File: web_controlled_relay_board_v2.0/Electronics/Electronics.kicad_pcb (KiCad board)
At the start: 2 copper layers, 165.2 x 114.6 mm, 71 parts, among them J1 Screw_Terminal_01x10, J2 Screw_Terminal_01x10, J3 Screw_Terminal_01x02, J4 Screw_Terminal_01x02, K1 G3MB-202P, K10 G3MB-202P, K11 G3MB-202P, K12 G3MB-202P, K13 G3MB-202P, K14 G3MB-202P, K15 G3MB-202P, K16 G3MB-202P, K17 G3MB-202P, K18 G3MB-202P, K19 G3MB-202P, K2 G3MB-202P, K20 G3MB-202P, K3 G3MB-202P, K4 G3MB-202P, K5 G3MB-202P, K6 G3MB-202P, K7 G3MB-202P, K8 G3MB-202P, K9 G3MB-202P, SW1 SW_MEC_5E, U1 PC817, U10 PC817, U11 PC817, U12 PC817, U13 PC817, U14 PC817, U15 PC817, U16 PC817, U17 PC817, U18 PC817, U19 PC817, U2 PC817, U20 PC817, U3 PC817, U4 PC817, U5 PC817, U6 PC817, U7 PC817, U8 PC817, U9 PC817

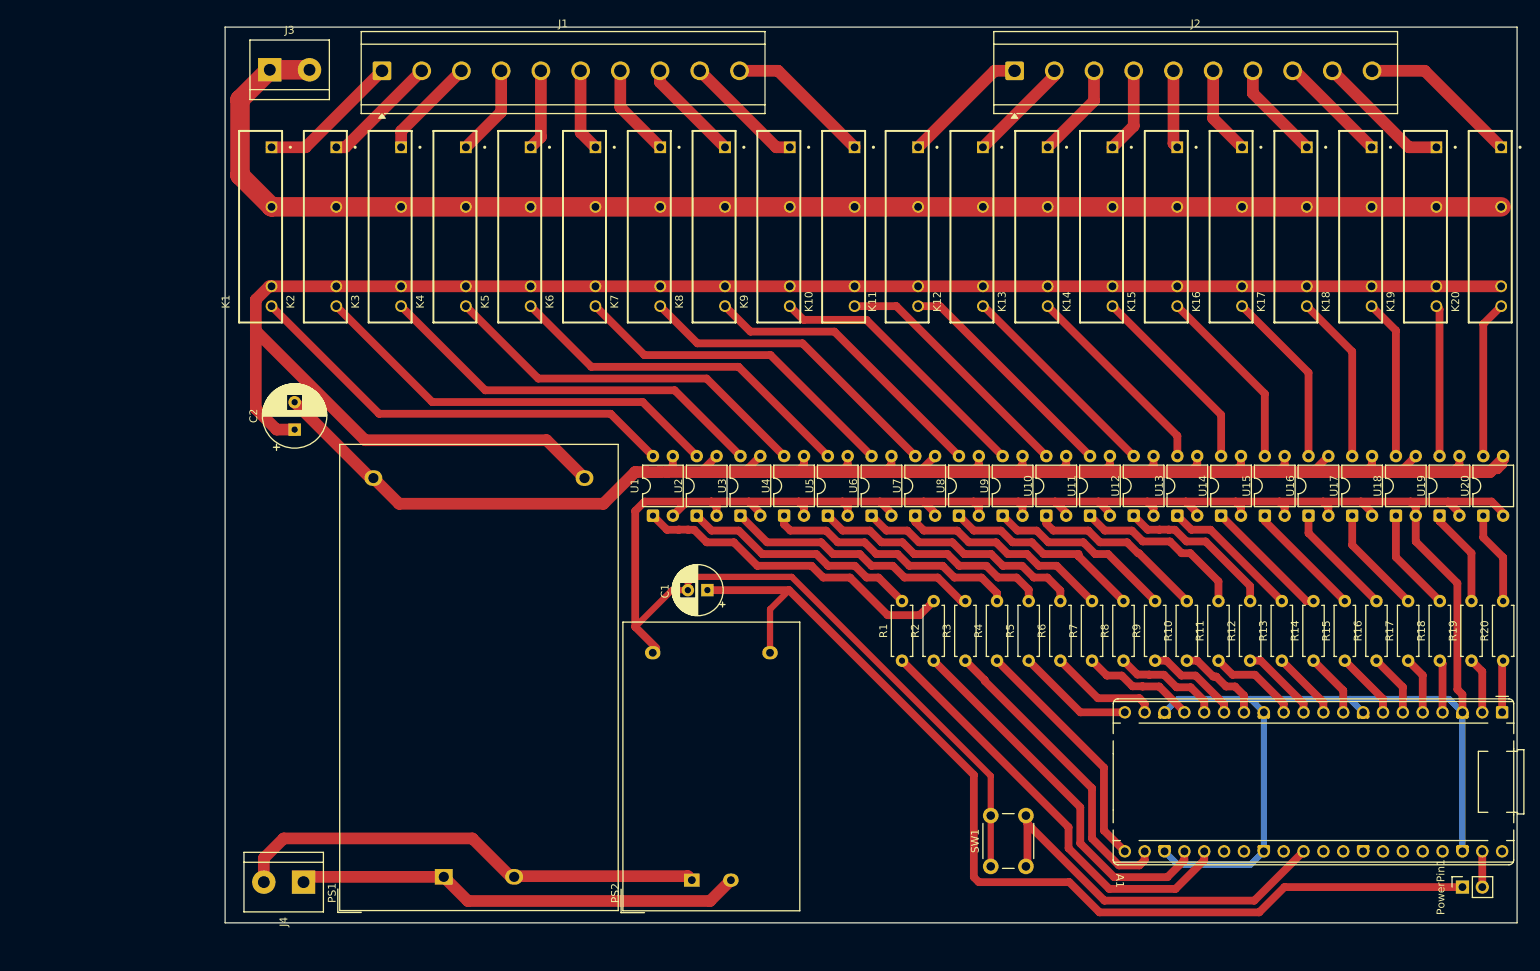
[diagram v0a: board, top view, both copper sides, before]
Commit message: bug fixes and added docs
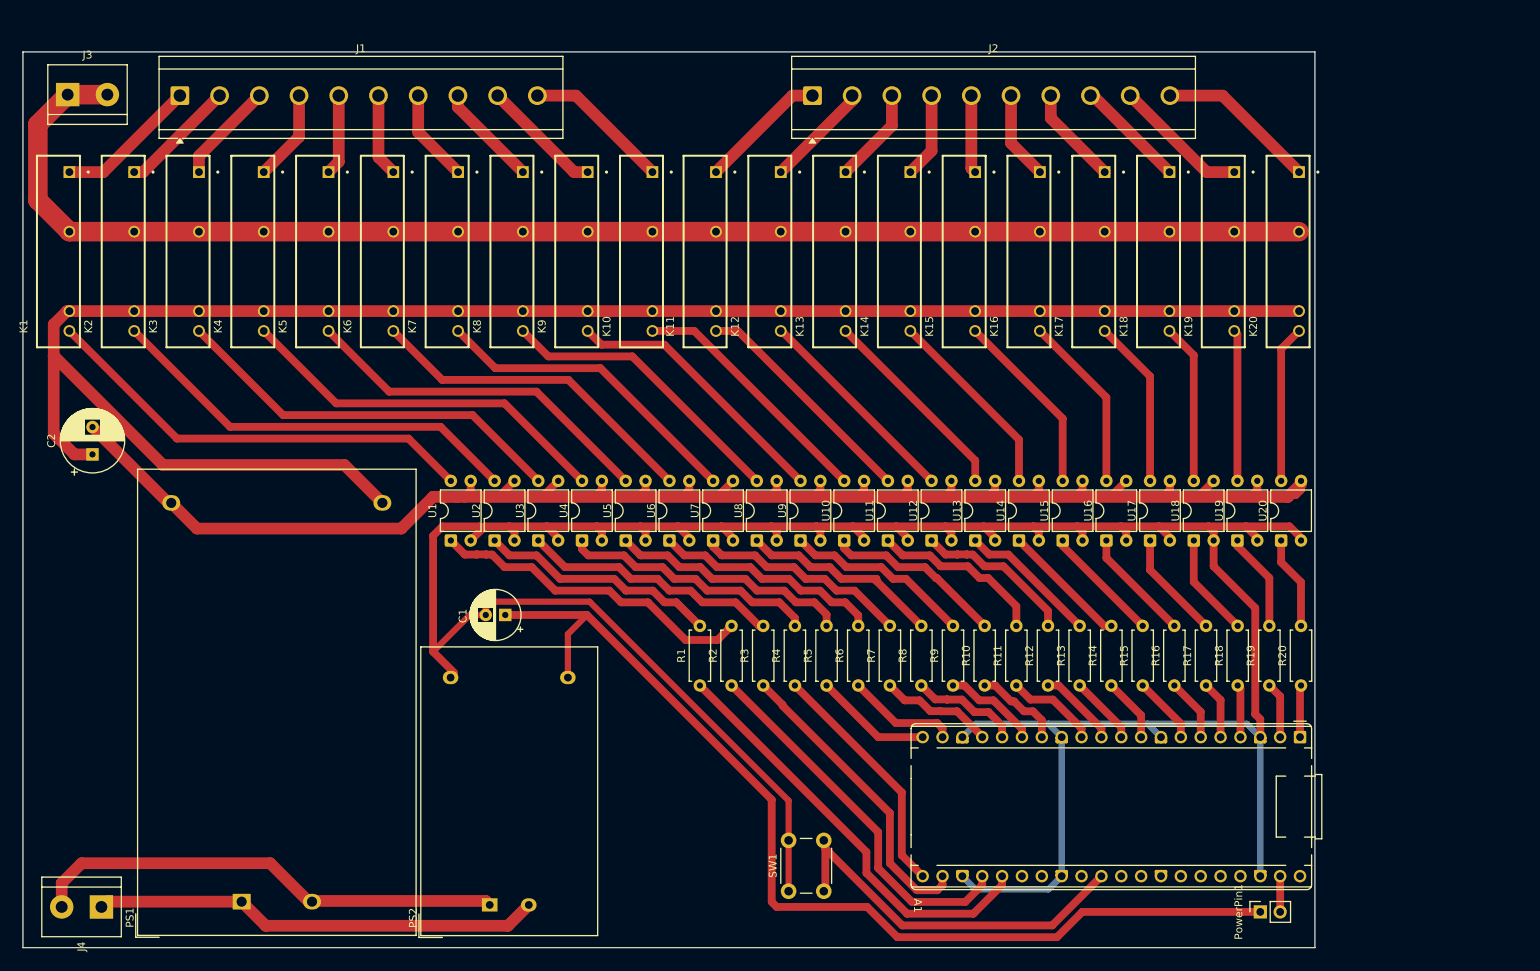
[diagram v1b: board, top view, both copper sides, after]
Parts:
- moved K16 26.0 mm to (155.1, 58.0)
- moved K17 26.0 mm to (163.4, 58.0)
- moved K18 26.0 mm to (171.7, 58.0)
- moved R11 26.0 mm to (153.5, 113.5)
- moved R13 26.0 mm to (161.6, 113.5)
- moved R16 26.0 mm to (173.7, 113.5)
- moved R19 26.0 mm to (185.9, 113.5)
- moved R6 26.0 mm to (133.3, 113.5)
- moved R8 26.0 mm to (141.4, 113.5)
- moved SW1 26.0 mm to (124.4, 139.8)
- moved U10 26.0 mm to (131.5, 95.0)
- moved U14 26.0 mm to (153.9, 95.0)
- moved U15 26.0 mm to (159.4, 95.0)
- moved C1 26.0 mm to (88.2, 104.5)
- moved K11 26.0 mm to (113.7, 58.0)
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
